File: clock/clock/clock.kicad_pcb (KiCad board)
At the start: 2 copper layers, 32.3 x 110 mm, 46 parts, among them J1 AVR-ISP, J10 Conn_01x07_Male, J11 CV_IN, J12 CLOCK_OUT, J13 SUBDIV_OUT, J2 EURORACK_CONN_10, J3 Conn_01x05_Female, J4 Conn_01x05_Male, J5 Conn_01x05_Female, J6 Conn_01x05_Male, J7 Conn_01x05_Female, J8 Conn_01x05_Male, J9 Conn_01x07_Female, SW1 SW_Push, SW2 SW_Push, SW3 Rotary_Encoder_Switch, U1 ATmega328P-PU, U2 L7805, U3 SM460281N, U4 SM460281N, U5 SM460281N, Y1 16MHz

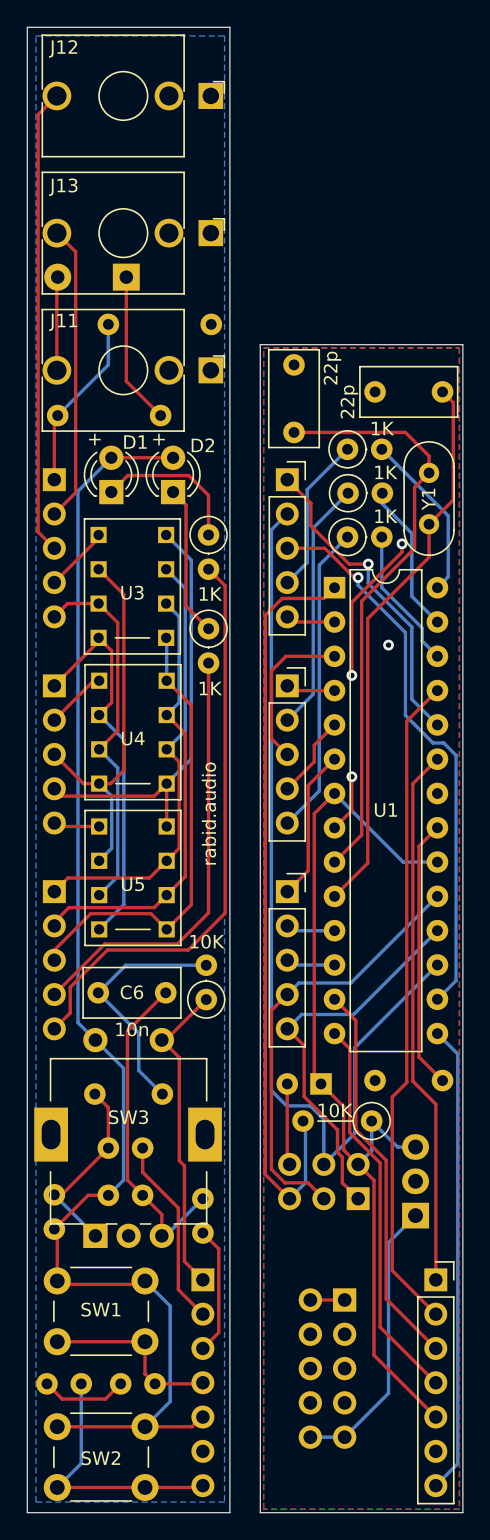
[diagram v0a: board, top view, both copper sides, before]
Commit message: make a bit more space
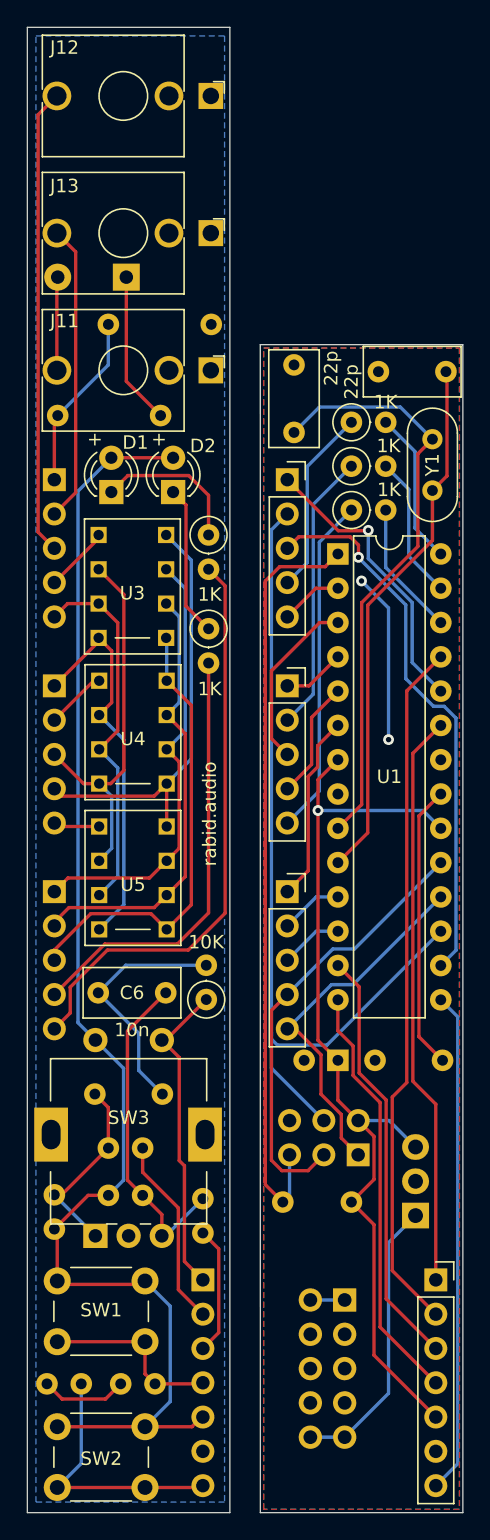
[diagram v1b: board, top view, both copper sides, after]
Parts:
- J1: value AVR-ISP -> ISP
- R1: moved to B.Cu
- moved R1 6.18 mm to (24.0, 87.0)
- moved J1 3.25 mm to (24.5, 83.5)
- moved U1 2.51 mm to (23.0, 39.0)
- moved Y1 2.51 mm to (30.0, 30.5)
- moved C1 2.15 mm to (23.0, 76.5)
- moved R6 2.02 mm to (24.0, 35.8)
- moved R8 2.02 mm to (24.0, 29.2)
- moved R7 2.02 mm to (24.0, 32.5)
- moved C4 1.52 mm to (26.0, 25.5)
- moved C2 1.50 mm to (25.8, 76.5)
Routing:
- net GND: track 21.6 -> 12.6 mm, vias 4 -> 2
- net /B_SUBDIV_OUT: track 70.7 -> 63.7 mm
- net /B_SW3: track 40.0 -> 42.6 mm
- net /B_LED3: track 6.18 -> 8.78 mm
- net /B_KNOBL: track 48.9 -> 51.5 mm
- net /B_KNOBR: track 29.0 -> 31.4 mm
- net /B_SW1: track 29.0 -> 31.4 mm
- net /B_LED4: track 11.7 -> 13.9 mm
- net /B_LED_C3: track 23.0 -> 25.1 mm
- net /B_LED_C1: track 11.7 -> 13.8 mm
- net /B_LED_C2: track 18.7 -> 20.8 mm
- net /B_CV_IN: track 24.3 -> 22.4 mm
- net Net-(R8-Pad2): track 13.2 -> 11.4 mm
- net /B_SW2: track 35.5 -> 37.2 mm
- net /B_LEDR: track 32.4 -> 34.0 mm
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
